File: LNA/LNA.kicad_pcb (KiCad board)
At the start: 2 copper layers, 19 parts, among them J1 SMA 50R, J2 SMA 50R, U1 SPF5189Z, U2 AMS1117-5.0

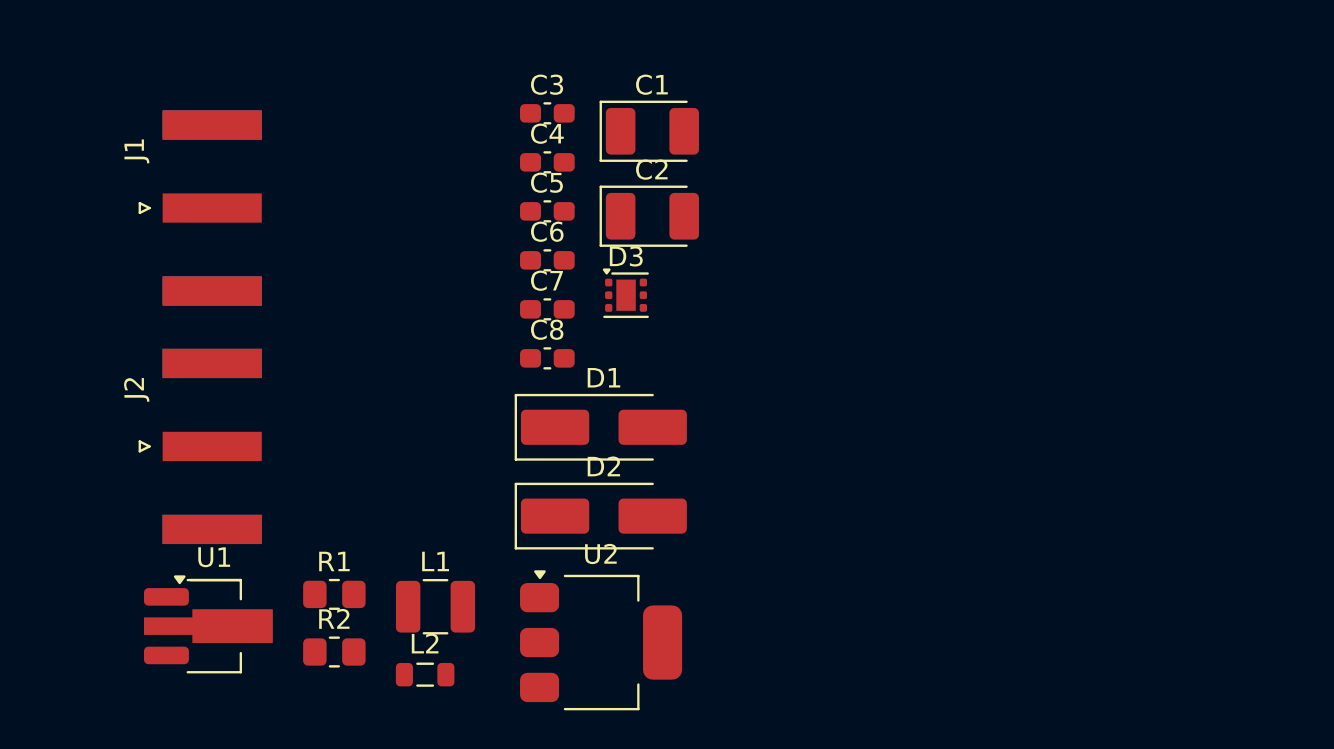
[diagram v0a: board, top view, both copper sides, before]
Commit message: finished routing
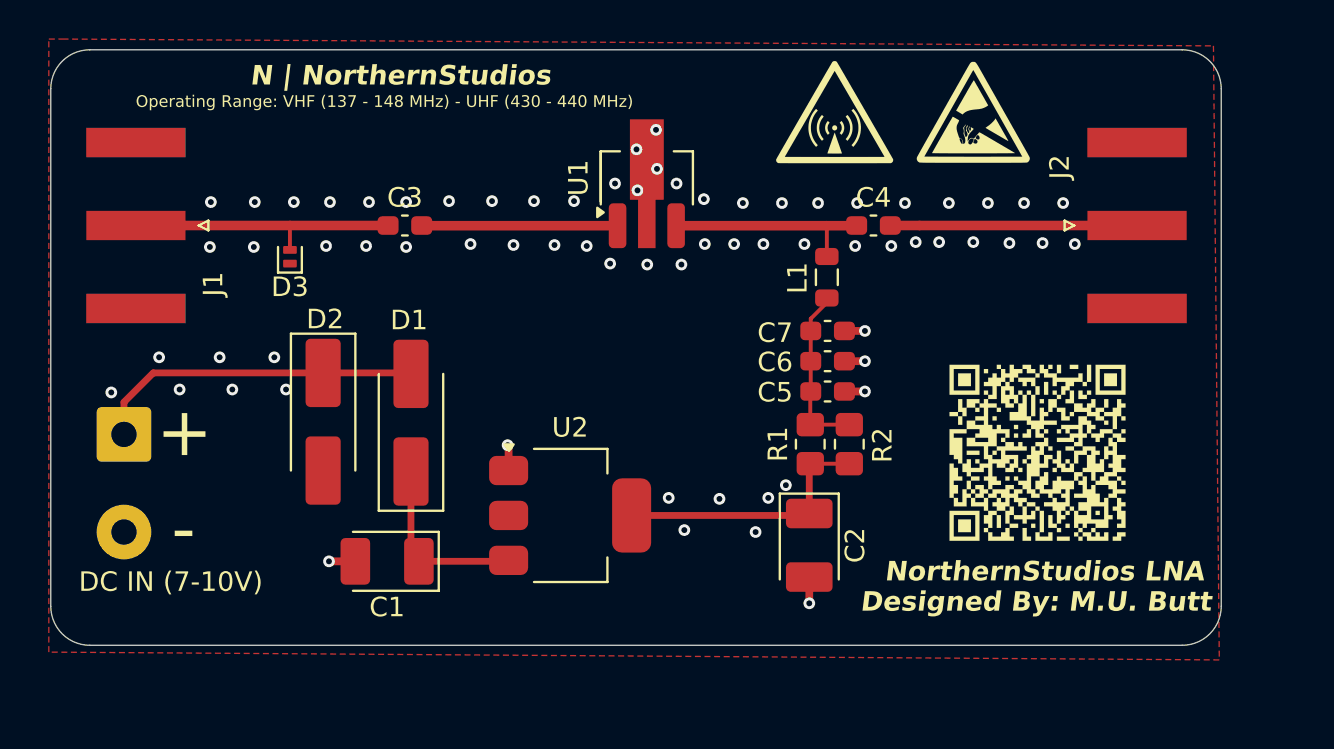
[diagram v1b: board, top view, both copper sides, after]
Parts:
- removed C8: 1uF, Capacitor_SMD:C_0603_1608Metric_Pad1.08x0.95mm_HandSolder
- removed L2: 330nH - 1uH, Inductor_SMD:L_0805_2012Metric
- added G***: LOGO, LOGO, F.Cu at (177.1, 93.7)
- added G***: LOGO, LOGO, F.Cu at (173.8, 76.2)
- added G***: LOGO, LOGO, F.Cu at (166.7, 76.2)
- added J3: DC IN (7-10V), TerminalBlock:TerminalBlock_MaiXu_MX126-5.0-02P_1x02_P5.00mm, F.Cu at (130.2, 92.7)
- D3: footprint Package_SON:WSON-6-1EP_2x2mm_P0.65mm_EP1x1.6mm -> Diode_SMD:D_SOD-882
- L1: value 10uH -> 470nH-1uH; footprint Inductor_SMD:L_1210_3225Metric -> Inductor_SMD:L_0805_2012Metric
- moved J2 48.7 mm to (182.1, 82.0)
- moved U1 31.9 mm to (157.0, 79.6), turned to 90 degrees
- moved R2 28.4 mm to (167.4, 93.2), turned to 90 degrees
- moved L1 26.2 mm to (166.2, 84.7), turned to 90 degrees
- moved C1 25.9 mm to (143.7, 99.2), turned to 180 degrees
- moved R1 25.6 mm to (165.4, 93.2), turned to 90 degrees
- moved C2 18.7 mm to (165.3, 98.4), turned to -90 degrees
- moved D3 17.3 mm to (138.8, 83.6), turned to 90 degrees
- moved C5 17.1 mm to (166.3, 90.5)
- moved C4 17.0 mm to (168.6, 82.0)
- moved C6 15.3 mm to (166.3, 89.0)
- moved D2 15.2 mm to (140.4, 92.0), turned to -90 degrees
- moved C7 14.4 mm to (166.3, 87.4)
- moved D1 9.88 mm to (144.9, 92.1), turned to 90 degrees
- moved C3 9.29 mm to (144.6, 82.0)
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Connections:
- L1 pad 2: Net-(C8-Pad1) -> Net-(C4-Pad1)
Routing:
- net Net-(D1-A): track 0.00 -> 17.1 mm
- net Net-(D3-A2): track 0.00 -> 14.2 mm
- net Net-(U2-VO): track 0.00 -> 13.9 mm
- net Net-(J2-In): track 0.00 -> 12.6 mm
- net Net-(C4-Pad1): track 0.00 -> 10.8 mm
- net Net-(C3-Pad2): track 0.00 -> 10.0 mm
- net Net-(D1-K): track 0.00 -> 9.45 mm
- net Net-(C5-Pad1): track 0.00 -> 8.84 mm
- net GND: track 0.00 -> 7.17 mm, vias 0 -> 69
- added copper zone on F.Cu, net GND
- added copper zone on In1.Cu, net GND
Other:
- board outline added: 59.9 x 30.5 mm
- copper layers 2 -> 4
- board text added: "+"
- board text added: "-"
- board text added: "Designed By: M.U. Butt"
- board text added: "N | NorthernStudios"
- board text added: "NorthernStudios LNA"
- board text added: "Operating Range: VHF (137 - 148 MHz) - UHF (430 - 440 MHz)"
